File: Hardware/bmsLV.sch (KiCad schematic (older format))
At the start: 28 parts, among them J1 Conn_01x06_Male, J2 USB_B_Mini, K1 RM85V7, Q1 BSS138, SW1 SW_Push, U1 STM32F103C8Tx, Y1 Crystal

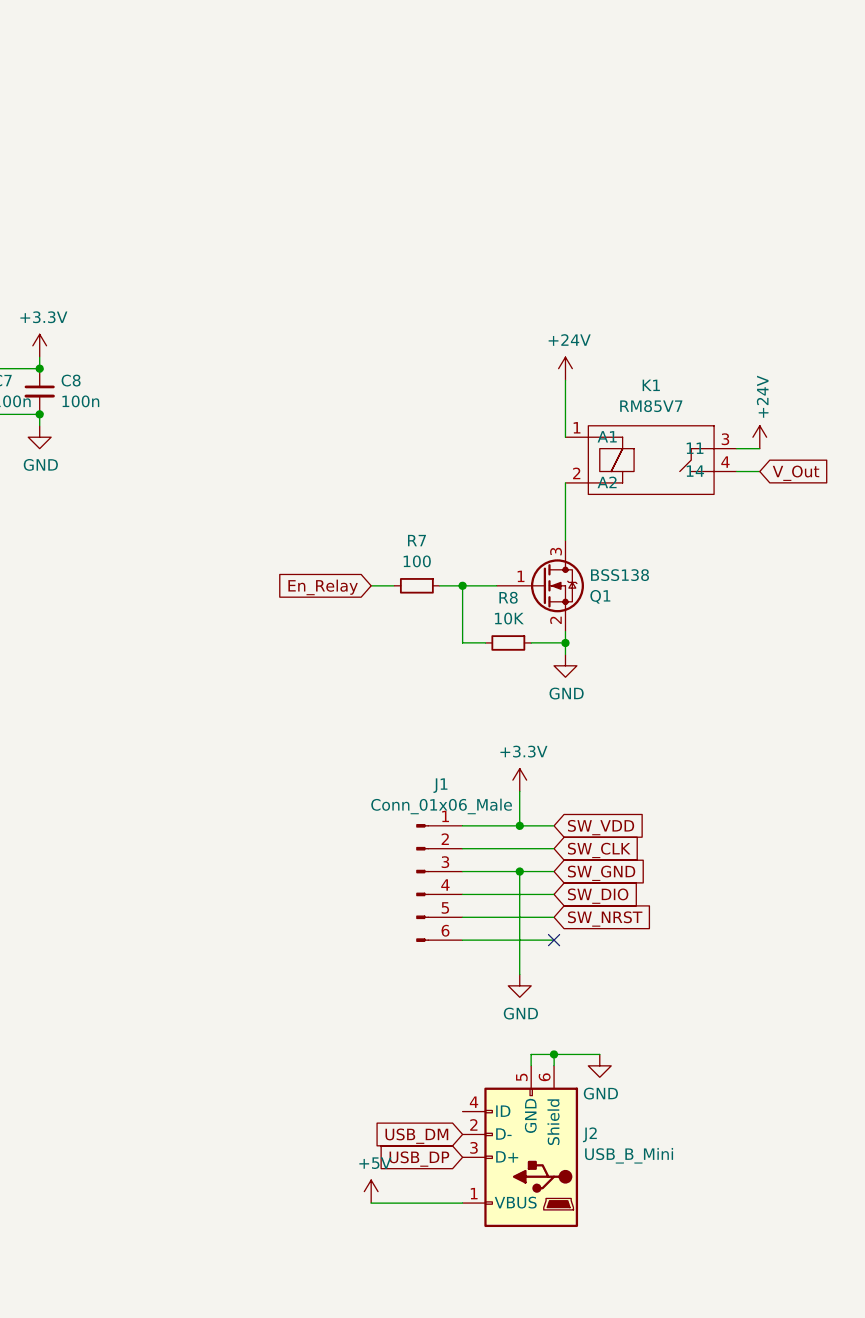
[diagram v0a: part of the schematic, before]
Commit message: Power update
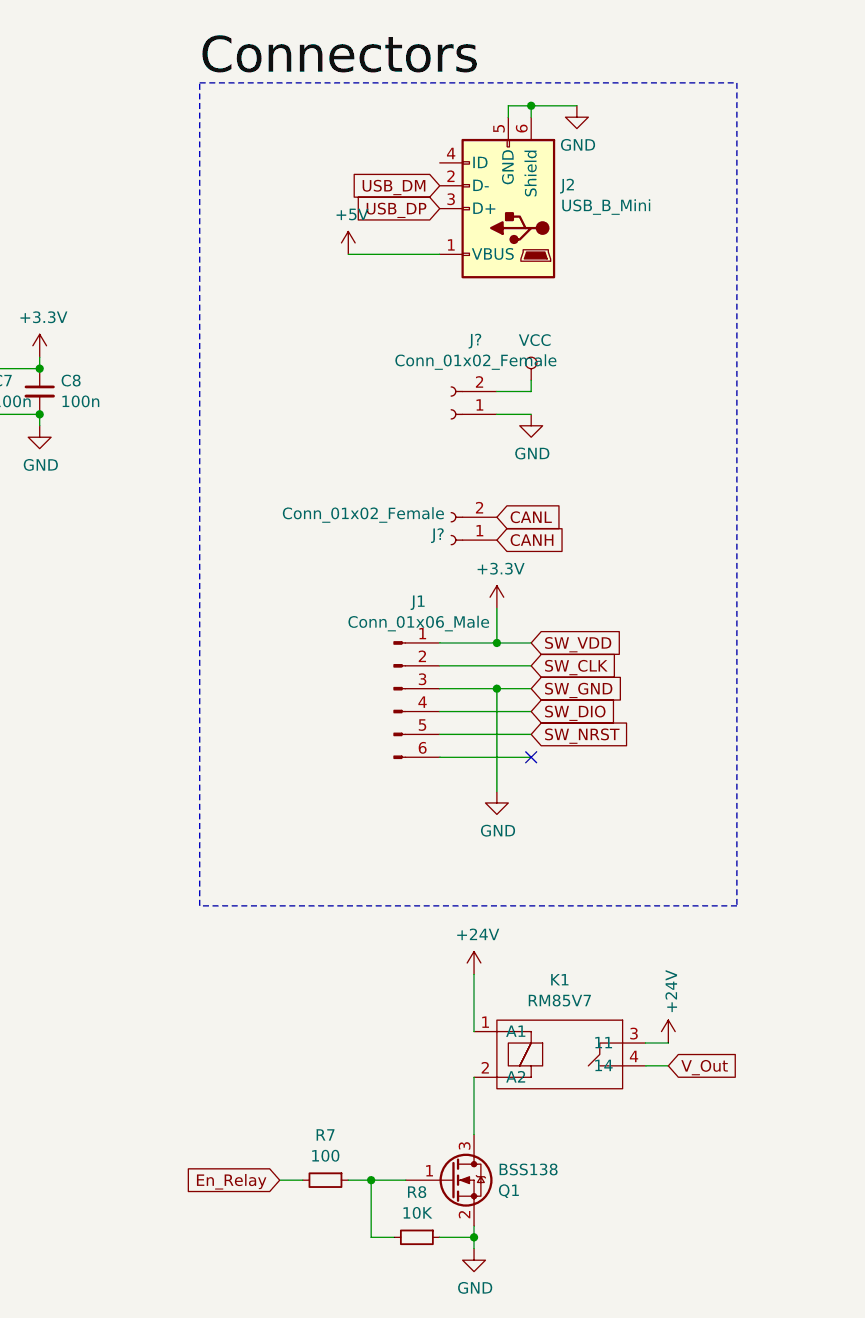
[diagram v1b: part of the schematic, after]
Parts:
- added J? (x2): Conn_01x02_Female, TerminalBlock:TerminalBlock_bornier-2_P5.08mm, symbol Connector:Conn_01x02_Female
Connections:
- net GND: now also J?.1 (Pin_1)
- new net CANH: J?.1 (Pin_1)
- new net CANL: J?.2 (Pin_2)
- new net VCC: J?.2 (Pin_2)
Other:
- moved on the sheet: J1, J2, K1, Q1, R7, R8
